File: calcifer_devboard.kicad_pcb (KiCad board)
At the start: 2 copper layers, 58.2 x 70.9 mm, 34 parts, among them J1 USB_C_Receptacle_USB2.0_14P, J2 Conn_01x03, J3 Conn_01x20, J4 Conn_01x20, SW1 SW_Push, U1 RP2040, U2 NCP1117-3.3_SOT223, U3 W25Q128JVS, Y1 23 MHz

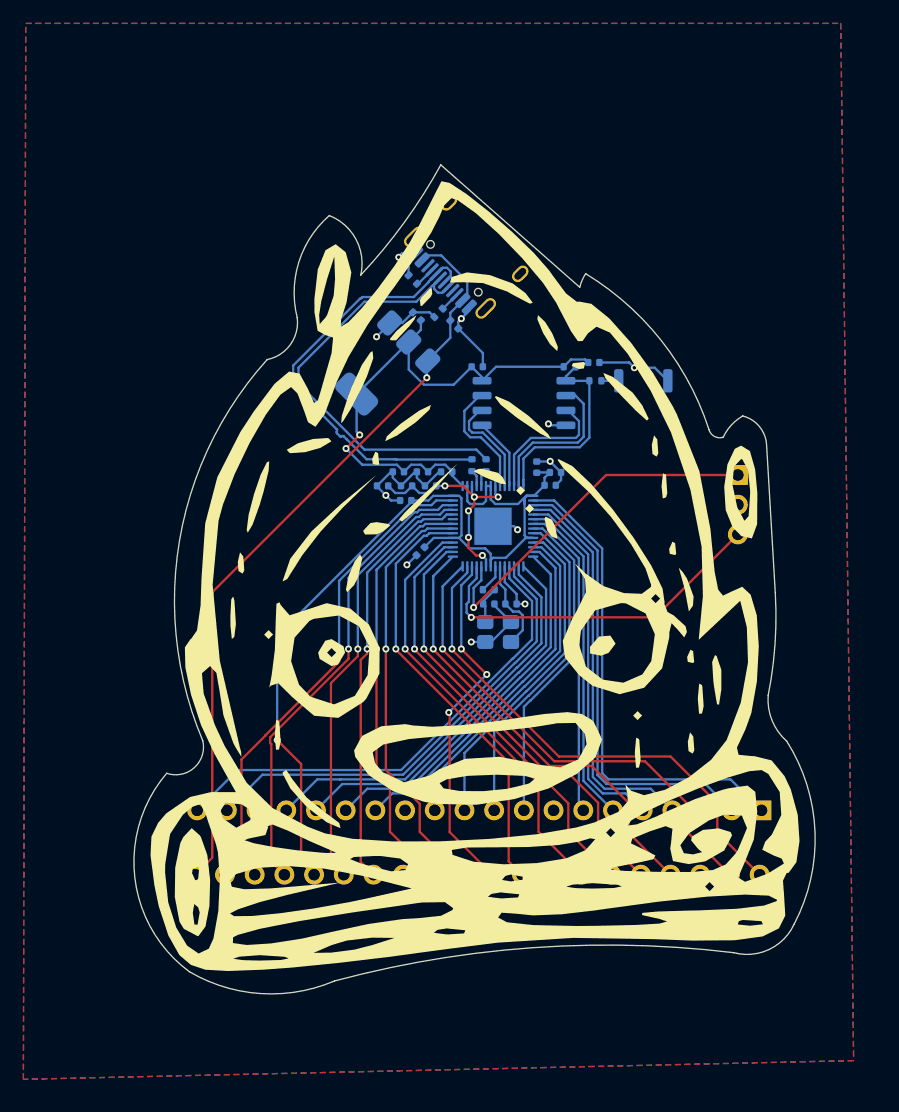
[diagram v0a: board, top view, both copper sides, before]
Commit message: retraced everything and finished readme
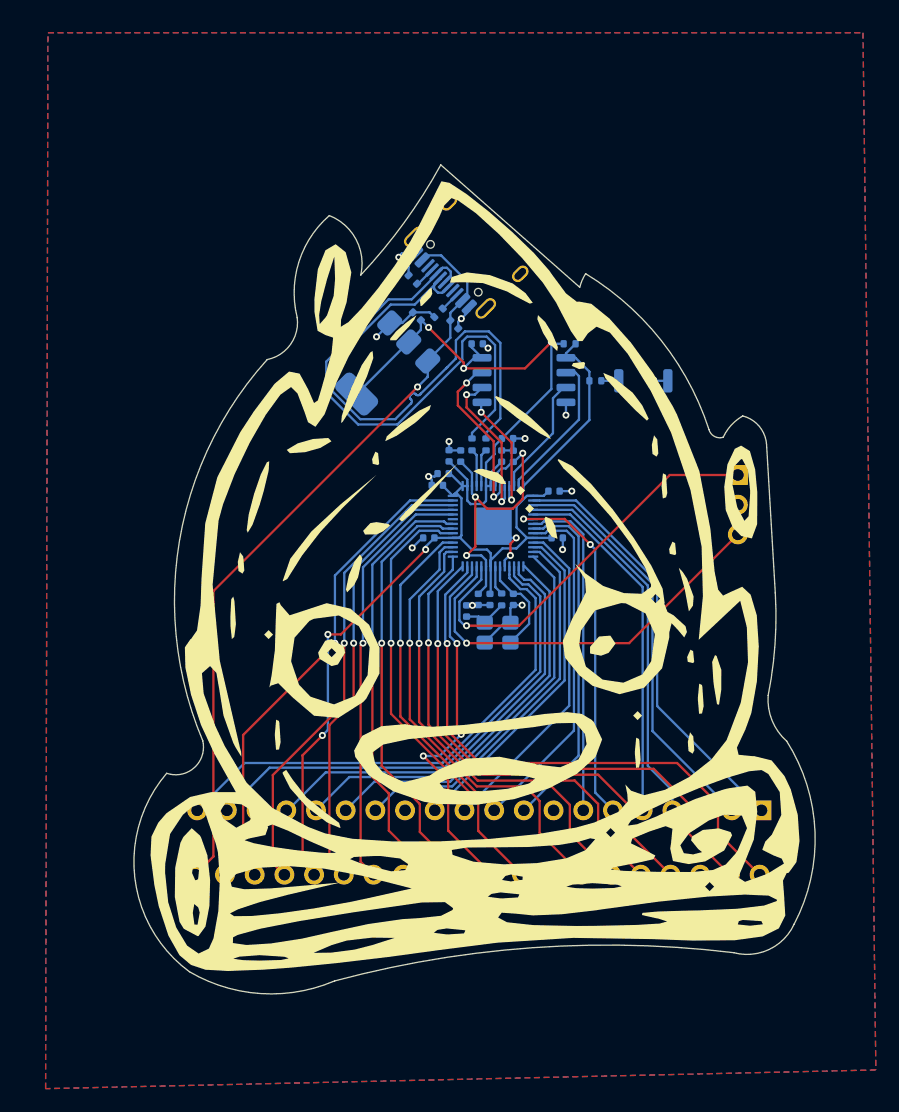
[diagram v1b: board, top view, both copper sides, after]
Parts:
- moved C6 15.3 mm to (137.8, 98.5)
- moved C8 12.2 mm to (132.0, 103.8), turned to -90 degrees
- moved C11 11.5 mm to (131.0, 103.8), turned to -90 degrees
- moved C10 11.5 mm to (134.0, 91.5), turned to 90 degrees
- moved C3 9.76 mm to (133.5, 90.0), turned to 0 degrees
- moved C12 3.63 mm to (129.5, 91.5), turned to 90 degrees
- moved C7 3.15 mm to (133.0, 91.5)
- moved C4 3.00 mm to (127.5, 94.0)
- moved C16 1.99 mm to (130.0, 104.8), turned to 90 degrees
- moved U3 1.97 mm to (134.9, 85.0)
- moved C17 1.96 mm to (130.9, 81.9)
- moved R4 1.96 mm to (138.8, 81.9)
- moved R6 1.78 mm to (131.7, 90.5)
- moved R7 1.78 mm to (130.5, 90.5)
- moved C2 1.78 mm to (128.0, 93.0)
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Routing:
- net GND: track 52.8 -> 37.2 mm, vias 11 -> 16
- net USB_D-: track 38.1 -> 46.6 mm
- net USB_D+: track 38.1 -> 46.6 mm
- net +3V3: track 124.6 -> 117.5 mm, vias 3 -> 6
- net +1V1: track 20.0 -> 26.6 mm, vias 6 -> 3
- net GPIO0: track 41.7 -> 36.7 mm
- net GPIO16: track 43.4 -> 48.2 mm
- net QSPI_SCLK: track 8.83 -> 13.4 mm, vias 0 -> 2
- net QSPI_SD0: track 6.16 -> 10.7 mm, vias 0 -> 2
- net GPIO17: track 41.8 -> 46.3 mm
- net GPIO18: track 38.4 -> 42.6 mm
- net SWD: track 30.6 -> 34.8 mm
- net GPIO19: track 38.1 -> 42.2 mm
- net GPIO20: track 36.7 -> 40.8 mm
- net QSPI_SD3: track 10.3 -> 14.3 mm, vias 0 -> 2
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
